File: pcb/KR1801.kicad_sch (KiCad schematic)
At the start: 1 part

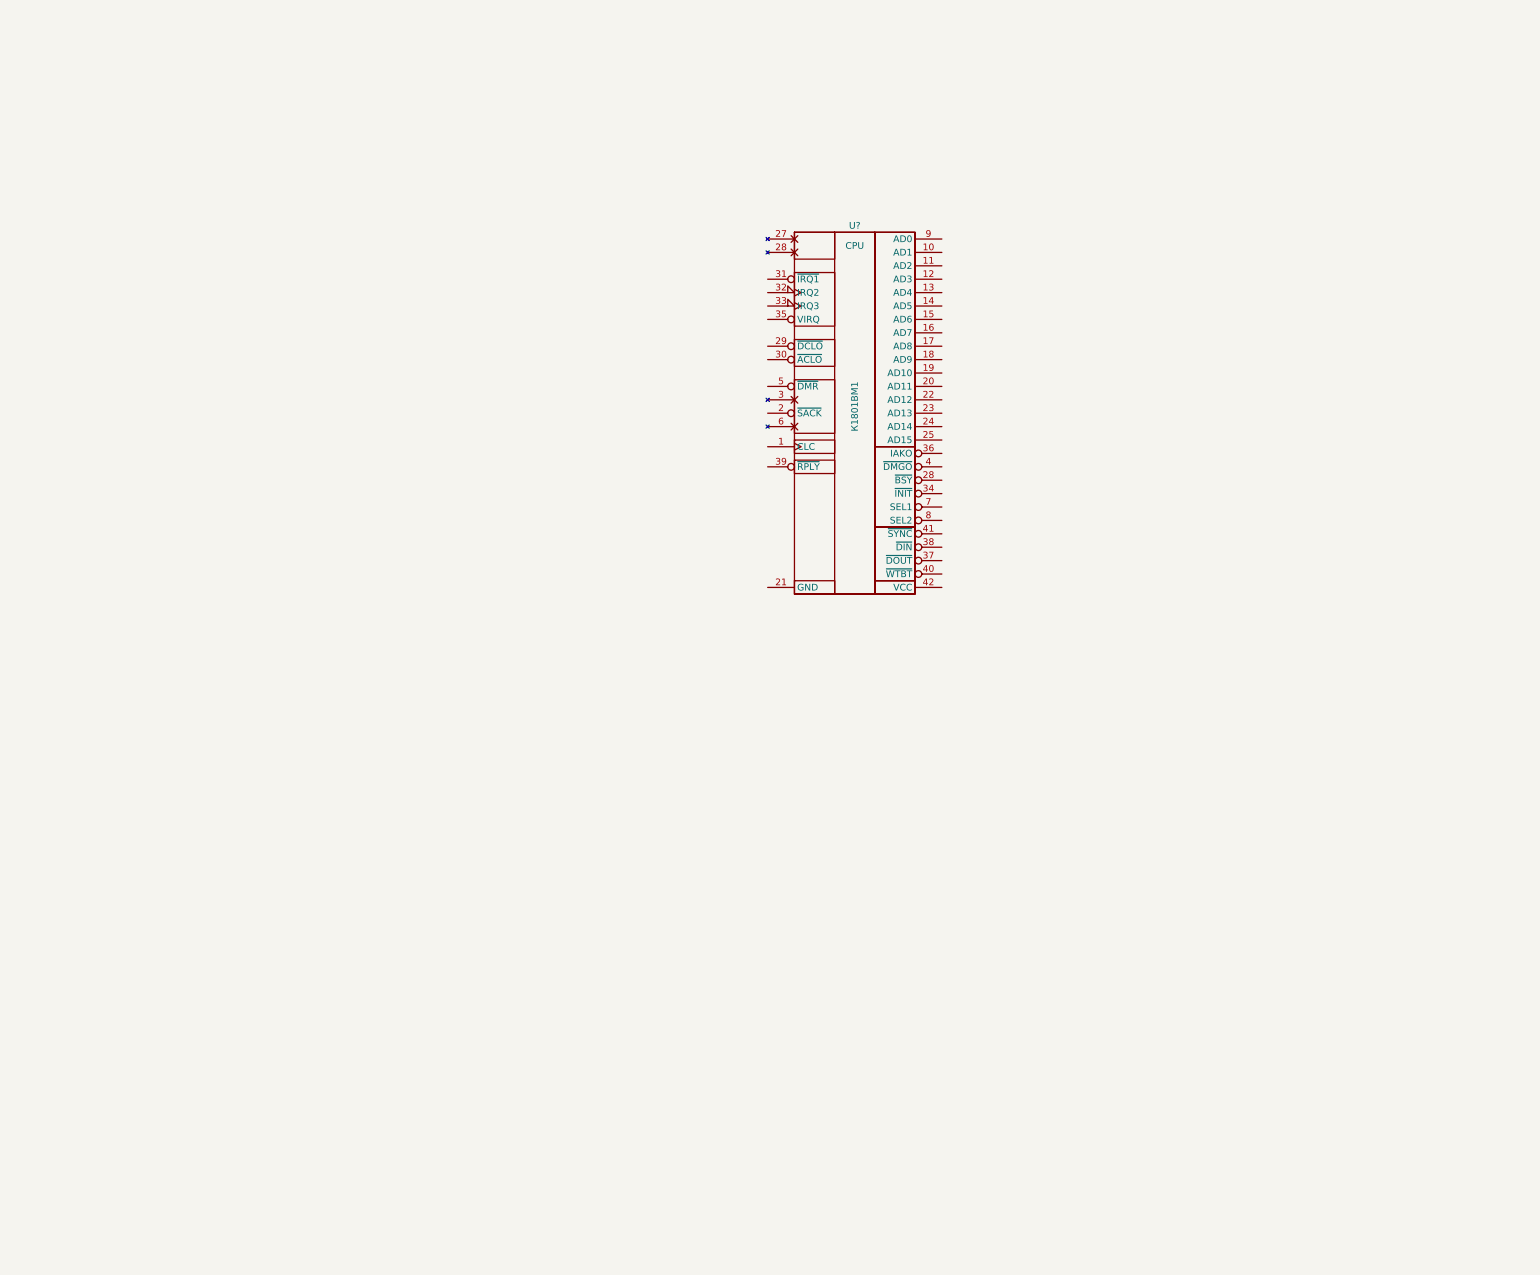
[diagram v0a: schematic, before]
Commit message: ECB
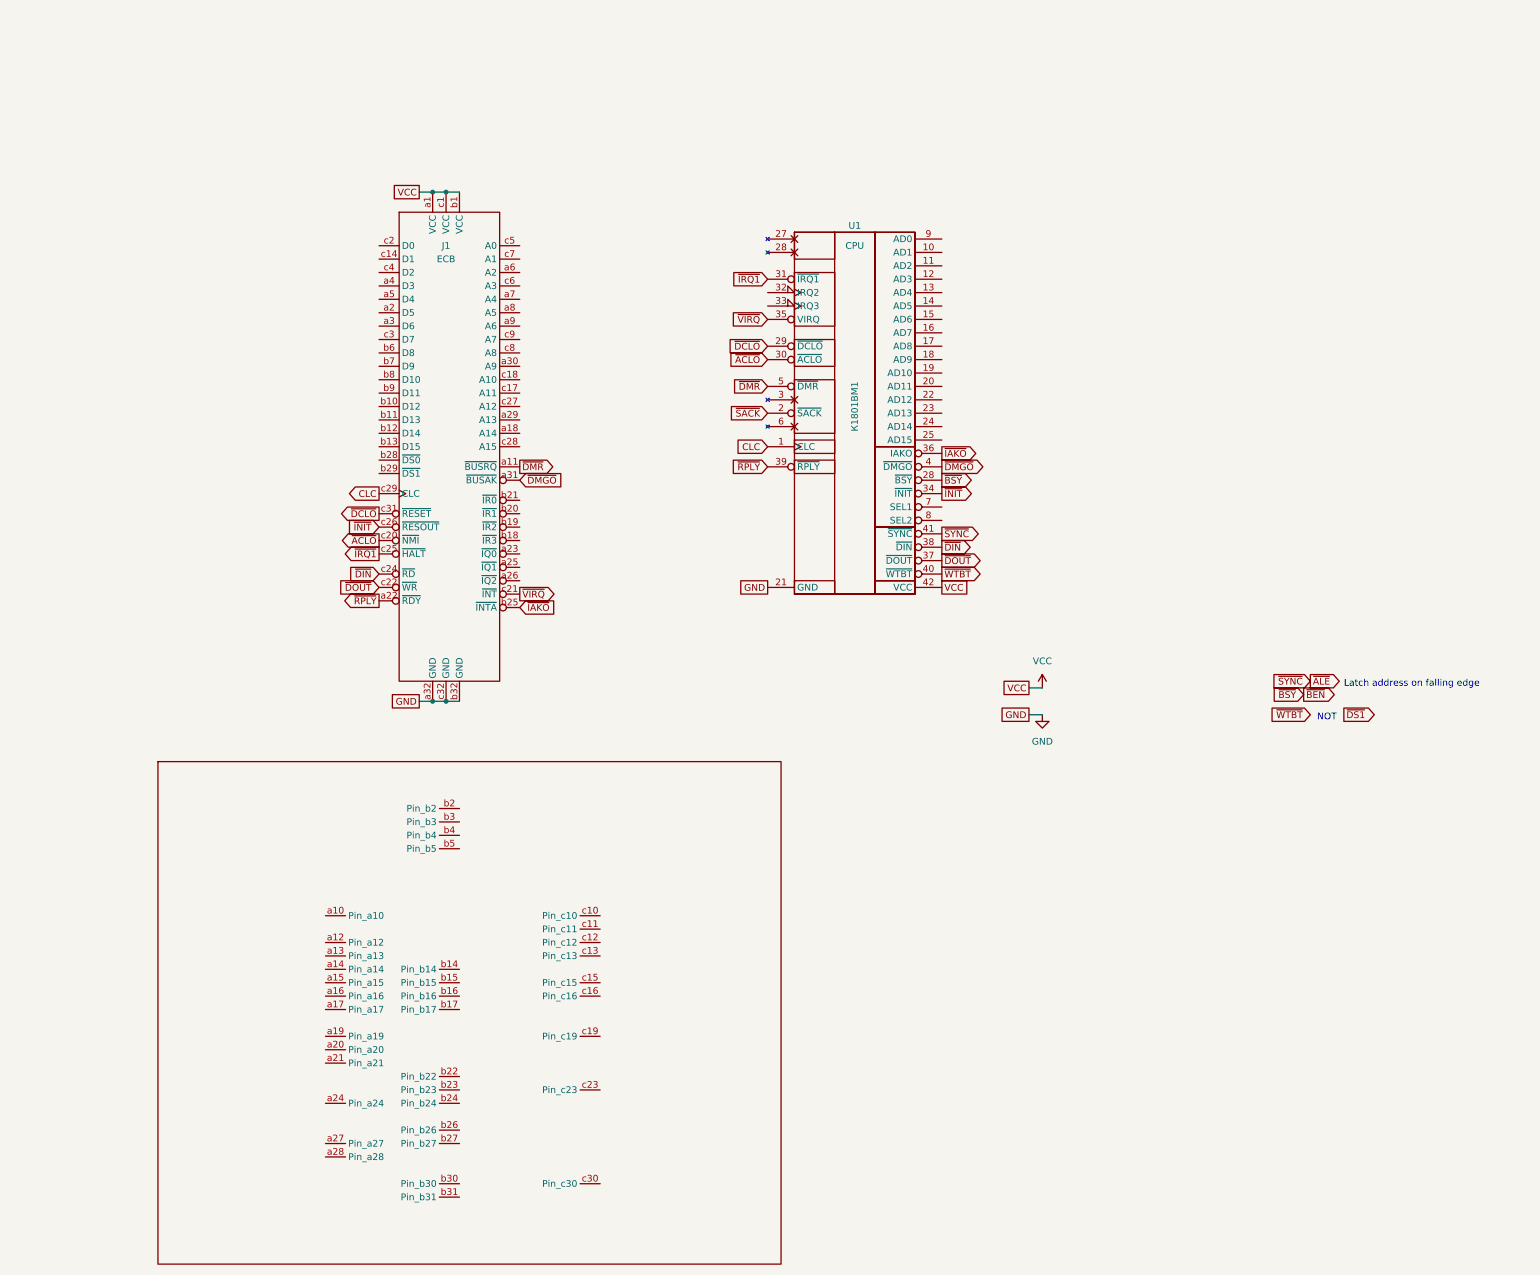
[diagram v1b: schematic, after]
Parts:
- added J1: ECB, Connector_DIN:DIN41612_R_3x32_Male_Horizontal_THT, symbol ECB:ECB_RB-6
- gave numbers to parts that had none: 1
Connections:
- net CLC: now reaches U1.1 (CLC)
- net CLC: now also J1.c29 (CLC)
- net ~{SACK}: now reaches U1.2 (~{SACK})
- net GND: now reaches U1.21 (GND)
- net GND: now also J1.a32 (GND), J1.b32 (GND), J1.c32 (GND)
- net ~{BEN}: now reaches U1.28 (~{BSY})
- net ~{DCLO}: now reaches U1.29 (~{DCLO})
- net ~{DCLO}: now also J1.c31 (~{RESET})
- net ~{ACLO}: now reaches U1.30 (~{ACLO})
- net ~{ACLO}: now also J1.c20 (~{NMI})
- net ~{IRQ1}: now reaches U1.31 (~{IRQ1})
- net ~{IRQ1}: now also J1.c25 (~{HALT})
- net ~{INIT}: now reaches U1.34 (~{INIT})
- net ~{INIT}: now also J1.c26 (~{RESOUT})
- net ~{VIRQ}: now reaches U1.35 (VIRQ)
- net ~{VIRQ}: now also J1.c21 (~{INT})
- net ~{IAKO}: now reaches U1.36 (IAKO)
- net ~{IAKO}: now also J1.b25 (~{INTA})
- net ~{DOUT}: now reaches U1.37 (~{DOUT})
- net ~{DOUT}: now also J1.c22 (~{WR})
- net ~{DIN}: now reaches U1.38 (~{DIN})
- net ~{DIN}: now also J1.c24 (~{RD})
- net ~{RPLY}: now reaches U1.39 (~{RPLY})
- net ~{RPLY}: now also J1.a22 (~{RDY})
- net ~{DMGO}: now reaches U1.4 (~{DMGO})
- net ~{DMGO}: now also J1.a31 (~{BUSAK})
- net ~{WTBT}: now reaches U1.40 (~{WTBT})
- net ~{ALE}: now reaches U1.41 (~{SYNC})
- net VCC: now reaches U1.42 (VCC)
- net VCC: now also J1.a1 (VCC), J1.b1 (VCC), J1.c1 (VCC)
- net ~{DMR}: now reaches U1.5 (~{DMR})
- net ~{DMR}: now also J1.a11 (~{BUSRQ})
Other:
- note added: "Latch address on falling edge"
- note added: "NOT"

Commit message: 3D models
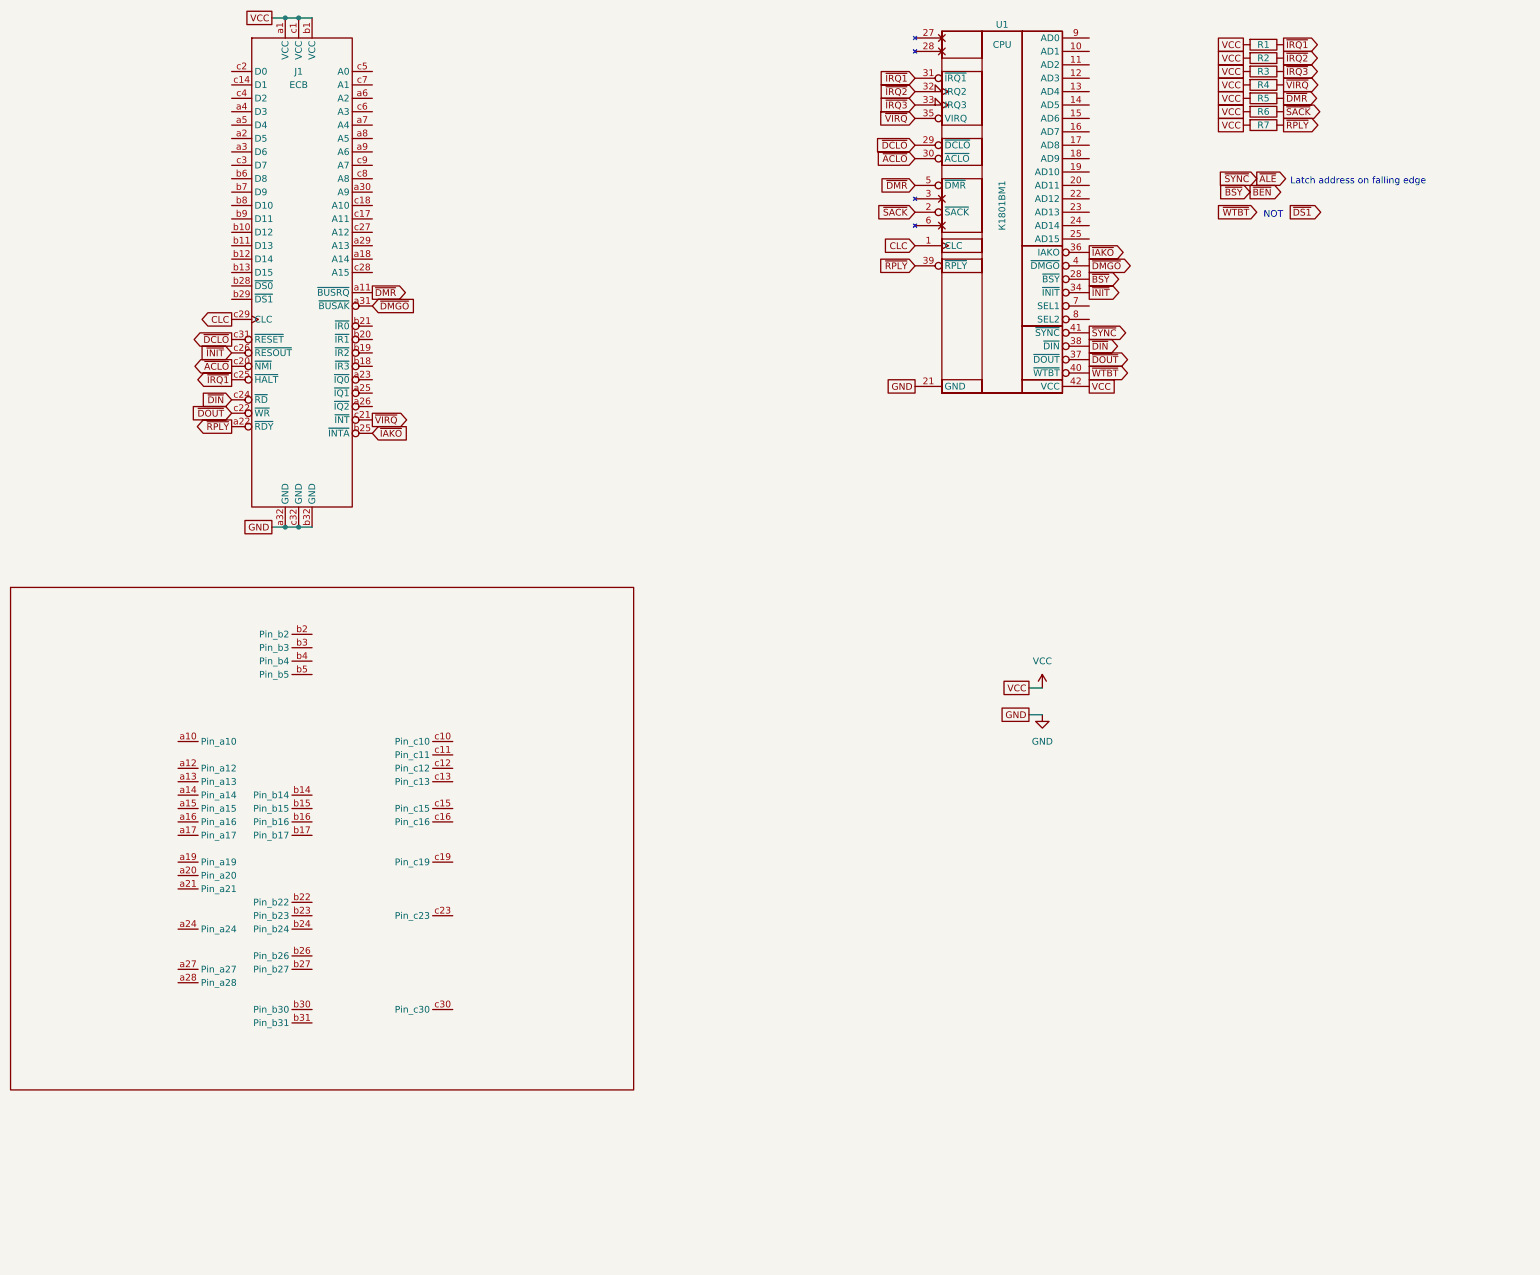
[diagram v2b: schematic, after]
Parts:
- added R1, R2, R3, R4, R5, R6, R7: R, symbol Device:R
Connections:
- net VCC: now also R1.2, R2.2, R3.2, R4.2, R5.2, R6.2, R7.2
- net ~{DMR}: now also R5.1
- net ~{IRQ1}: now also R1.1
- net ~{RPLY}: now also R7.1
- net ~{SACK}: now also R6.1
- net ~{VIRQ}: now also R4.1
- net ~{IRQ2}: now reaches U1.32 (IRQ2)
- net ~{IRQ2}: now also R2.1
- net ~{IRQ3}: now reaches U1.33 (IRQ3)
- net ~{IRQ3}: now also R3.1
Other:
- moved on the sheet: J1, U1

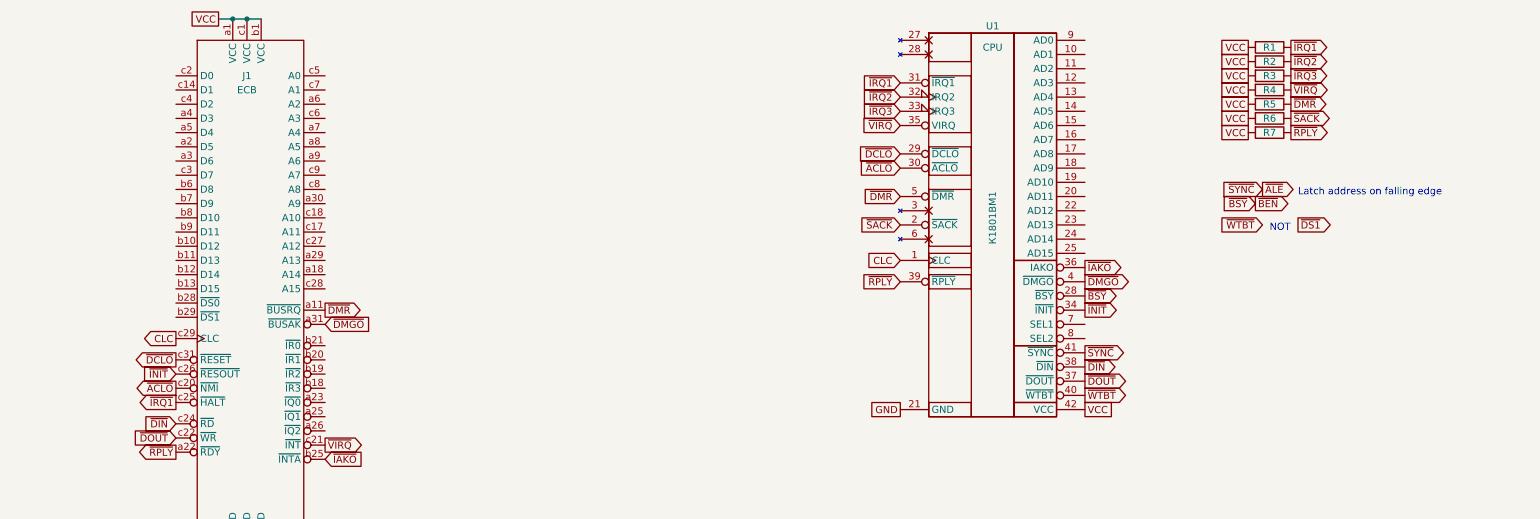
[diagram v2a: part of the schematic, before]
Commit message: more docs and boot
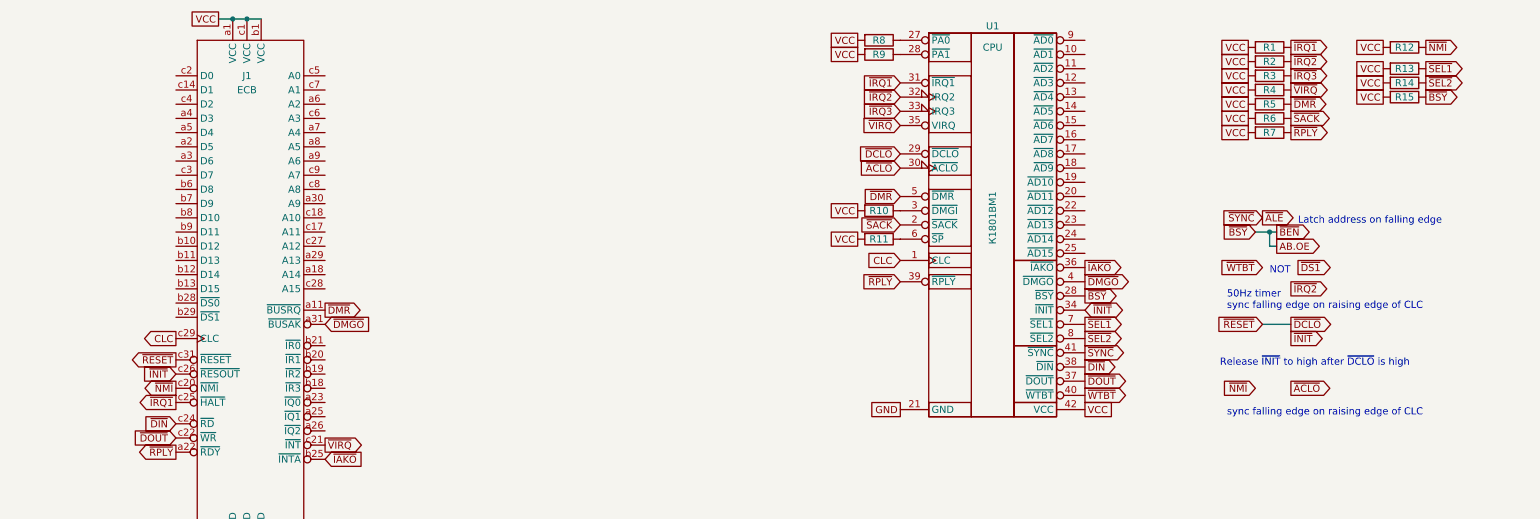
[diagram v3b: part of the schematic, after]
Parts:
- added R10, R11, R9: 0R, symbol Device:R
- added R12, R13, R14, R15: R, symbol Device:R
- added R8: OR, symbol Device:R
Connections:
- net ~{BEN} is gone; now on net AB.OE: U1.28 (~{PA1})
- net VCC: now also R10.2, R11.2, R12.2, R13.2, R14.2, R15.2, R8.2, R9.2
- net ~{ACLO}: no longer J1.c20 (~{NMI})
- net at U1.27 (~{PA0}): now also R8.1
- net AB.OE: now reaches U1.28 (~{PA1})
- net AB.OE: now also R15.1
- net at U1.3 (~{DMGI}): now also R10.1
- net at U1.6 (~{SP}): now also R11.1
- net ~{SEL1}: now reaches U1.7 (~{SEL1})
- net ~{SEL1}: now also R13.1
- net ~{SEL2}: now reaches U1.8 (~{SEL2})
- net ~{SEL2}: now also R14.1
- new net: R9.1, U1.28 (~{PA1})
- new net ~{NMI}: J1.c20 (~{NMI}), R12.1
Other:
- note added: "50Hz timer sync falling edge on raising edge of CLC"
- note added: "Release ~{INIT} to high after ~{DCLO} is high"
- note added: "sync falling edge on raising edge of CLC"
